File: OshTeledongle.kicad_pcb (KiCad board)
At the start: 4 copper layers, 25 x 57.5 mm, 62 parts, among them J2 Conn_ARM_SWD_TagConnect_TC203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, J3 SMA_Edgelaunch, J4 USB_C_Receptacle_USB2.0_16P, U1 AP2112K-3.3, U2 WE-TVS-82400102, U3 STM32F042C4Tx, U4 RN4678-V/RM113, U8 CC1200, Y1 ABM8W-40.0000MHZ, Y2 ECS-320-8-33Q-JES-TR

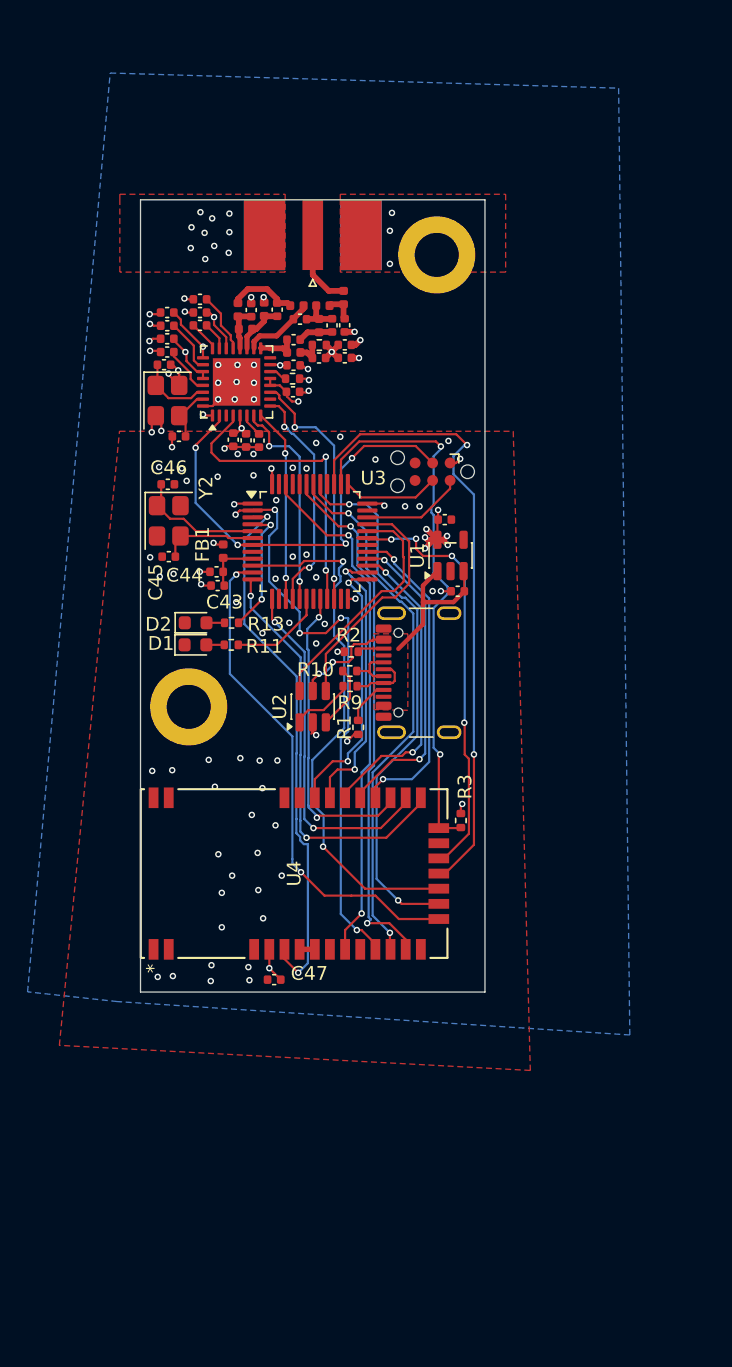
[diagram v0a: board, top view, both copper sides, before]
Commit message: v1.0 sent to fab
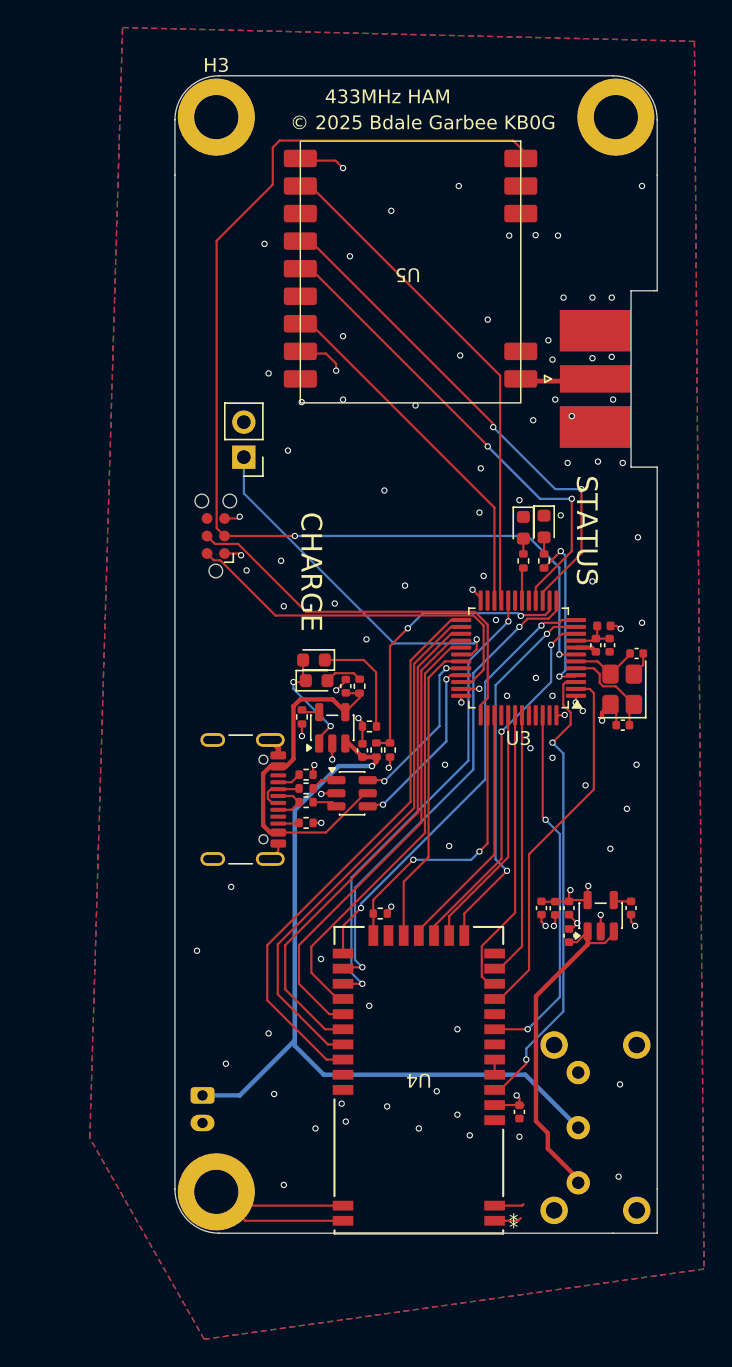
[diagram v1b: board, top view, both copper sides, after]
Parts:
- removed C11, C12, C14, C15, C28, C29, C30, C32, C34: 47nF, Capacitor_SMD:C_0402_1005Metric
- removed C13: 0.22uF, Capacitor_SMD:C_0402_1005Metric
- removed C25, C26: 10pF, Capacitor_SMD:C_0402_1005Metric
- removed C27: 1.8nF, Capacitor_SMD:C_0402_1005Metric
- removed C31: 56pF, Capacitor_SMD:C_0402_1005Metric
- removed C33, C35: 10nF, Capacitor_SMD:C_0402_1005Metric
- removed C36: 100pF, Capacitor_SMD:C_0402_1005Metric
- removed C37, C38, C39: 5.1pF, Capacitor_SMD:C_0402_1005Metric
- removed C40: 39pF, Capacitor_SMD:C_0402_1005Metric
- removed C41: 2.2pF, Capacitor_SMD:C_0402_1005Metric
- removed C42: 6.2pF, Capacitor_SMD:C_0402_1005Metric
- removed L1, L2: LQG15HS56NJ02D, Inductor_SMD:L_0402_1005Metric
- removed L3, L4: LQG15HZ27NJ02D, Inductor_SMD:L_0402_1005Metric
- removed L5, L6: LQG15HS15NJ02D, Inductor_SMD:L_0402_1005Metric
- removed L7: MLG1005S43NJTD25, Inductor_SMD:L_0402_1005Metric
- removed L8: LQG15HS22NG02D, Inductor_SMD:L_0402_1005Metric
- removed R12: 56k, Resistor_SMD:R_0402_1005Metric
- removed R48: 18, Resistor_SMD:R_0402_1005Metric
- removed U1: AP2112K-3.3, Package_TO_SOT_SMD:SOT-23-5
- removed U8: CC1200, Package_DFN_QFN:QFN-32-1EP_5x5mm_P0.5mm_EP3.45x3.45mm
- removed Y1: ABM8W-40.0000MHZ, Crystal:Crystal_SMD_Abracon_ABM8G-4Pin_3.2x2.5mm
- added C20: 4.7uF, Capacitor_SMD:C_0402_1005Metric, F.Cu at (52.4, 60.3)
- added C21: 4.7uF, Capacitor_SMD:C_0402_1005Metric, F.Cu at (53.6, 65.0)
- added C24: 1uF, Capacitor_SMD:C_0402_1005Metric, F.Cu at (68.6, 76.4)
- added C3: 100nF, Capacitor_SMD:C_0402_1005Metric, F.Cu at (67.6, 76.4)
- added C4: 10nF, Capacitor_SMD:C_0402_1005Metric, F.Cu at (73.1, 76.4)
- added D3: LED, LED_SMD:LED_0603_1608Metric, F.Cu at (50.1, 58.4)
- added D4: LED, LED_SMD:LED_0603_1608Metric, F.Cu at (50.3, 59.9)
- added G***: LOGO, LOGO, B.Cu at (59.9, 38.1)
- added G***: LOGO, LOGO, B.Cu at (58.0, 82.0)
- added H3: MountingHole_Pad, MountingHole:MountingHole_3.2mm_M3_DIN965_Pad, F.Cu at (43.0, 19.0)
- added J1: SMA_Edgelaunch, Connector_Coaxial:SMA_Amphenol_132289_EdgeMount, F.Cu at (70.5, 38.0)
- added J5: Conn_01x02, Connector_PinHeader_2.54mm:PinHeader_1x02_P2.54mm_Vertical, F.Cu at (45.0, 43.7)
- added R37: 2.49k, Resistor_SMD:R_0402_1005Metric, F.Cu at (49.2, 62.5)
- added R4: 1k, Resistor_SMD:R_0402_1005Metric, F.Cu at (53.4, 60.3)
- added R5: 1k, Resistor_SMD:R_0402_1005Metric, F.Cu at (54.1, 63.2)
- added R6: 10k, Resistor_SMD:R_0402_1005Metric, F.Cu at (55.6, 64.9)
- added R7: 5.1k, Resistor_SMD:R_0402_1005Metric, F.Cu at (54.6, 64.9)
- added SW1: SW_Push_SPDT, Button_Switch_THT:SW_E-Switch_EG1224_SPDT_Angled, B.Cu at (69.3, 88.3)
- added U17: MCP73831-2-OT, Package_TO_SOT_SMD:SOT-23-5, F.Cu at (51.4, 63.3)
- added U18: AP131-33, Package_TO_SOT_SMD:SOT-23-5, F.Cu at (70.9, 77.0)
- added U5: ~, FCU2025Lib:N511CS, F.Cu at (65.1, 20.7)
- C2: value 1uF -> 100nF
- J3: value SMA_Edgelaunch -> Conn_01x02; footprint Connector_Coaxial:SMA_Amphenol_132289_EdgeMount -> Connector_JST:JST_PH_S2B-PH-K_1x02_P2.00mm_Horizontal; moved to B.Cu
- moved J3 63.0 mm to (42.0, 90.0), turned to -90 degrees
- moved C46 37.4 mm to (72.5, 63.1), turned to 0 degrees
- moved H2 35.3 mm to (43.0, 97.0)
- moved Y2 35.1 mm to (72.5, 60.5), turned to 90 degrees
- moved C45 34.7 mm to (73.5, 57.9), turned to 180 degrees
- moved C2 29.0 mm to (66.6, 76.4), turned to 90 degrees
- moved C44 29.0 mm to (71.5, 57.3), turned to 90 degrees
- moved FB1 28.2 mm to (71.1, 55.9), turned to 180 degrees
- moved C43 27.8 mm to (70.5, 57.3), turned to 90 degrees
- moved C1 26.3 mm to (68.6, 78.4), turned to -90 degrees
- moved D2 26.2 mm to (66.8, 48.7), turned to -90 degrees
- moved D1 25.3 mm to (65.3, 48.8), turned to -90 degrees
- moved R13 23.1 mm to (66.8, 51.2), turned to -90 degrees
- moved R11 22.1 mm to (65.3, 51.2), turned to -90 degrees
- moved C47 20.2 mm to (65.0, 91.2), turned to -90 degrees
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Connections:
- C1 pad 2: VBUS -> Net-(SW1-C)
- J3 pad 1: Net-(J3-In) -> V_CHARGE
- U3 pad 14: /VDIV -> /V_BATT
- U3 pad 30: unconnected-(U3-PA9-Pad30) -> Net-(J5-Pin_1)
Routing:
- net V_CHARGE: track 0.00 -> 59.1 mm, vias 0 -> 1
- net /NRST: track 33.1 -> 82.6 mm, vias 4 -> 2
- net /BT_P2_0: track 46.1 -> 18.3 mm, vias 2 -> 0
- net Net-(J5-Pin_1): track 0.00 -> 26.2 mm, vias 0 -> 1
- net Net-(SW1-C): track 0.00 -> 25.9 mm
- net /SWCLK: track 7.06 -> 29.8 mm
- net /SCK2: track 14.1 -> 36.3 mm
- net GND: track 28.0 -> 50.1 mm, vias 102 -> 95
- net /BT_P0_5: track 39.7 -> 17.8 mm, vias 2 -> 0
- net /BT_P3_7: track 19.5 -> 41.1 mm, vias 2 -> 0
- net /V_BATT: track 0.00 -> 21.6 mm, vias 0 -> 2
- net +3V3: track 37.7 -> 17.6 mm, vias 21 -> 11
- net /SWDIO: track 7.46 -> 27.4 mm
- net /BT_P1_2: track 38.7 -> 19.4 mm, vias 2 -> 0
- net /BT_NRST: track 40.5 -> 21.9 mm
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- removed copper zone on F.Cu, net VBUS
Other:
- board size 25 x 57.5 mm -> 35 x 84 mm
- board text added: "+ -"
- board text added: "433MHz HAM"
- board text added: "CHARGE"
- board text added: "Leviathan Flight Systems K.Zheng"
- board text added: "RE-leBT v1.0"
- board text added: "STATUS"
- board text added: "© 2025 Bdale Garbee KB0G"
